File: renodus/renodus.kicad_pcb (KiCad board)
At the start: 4 copper layers, 40 x 40 mm, 67 parts, among them J1 USB_C_Receptacle_PowerOnly_6P, J2 Conn_01x02_Socket, J3 Conn_ARM_SWD_TagConnect_TC2030, SW1 SW_Push, SW2 SW_Push, U1 nRF54lxx_QDAA, U2 NPM1300-QEAA-R, U3 SHT4x, U4 STCC4, Y1 Crystal_GND24_Small, Y2 Crystal_Small

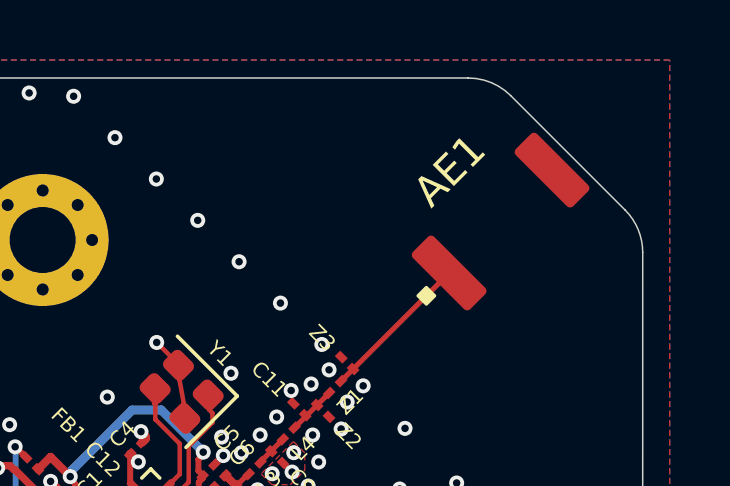
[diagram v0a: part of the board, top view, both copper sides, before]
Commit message: Small update
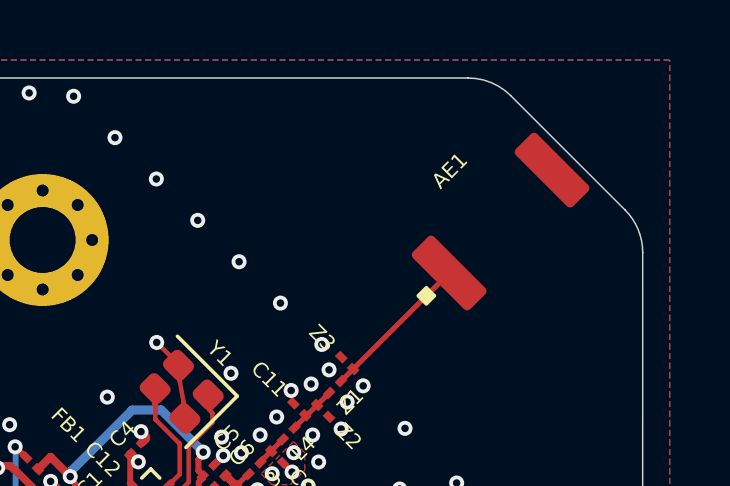
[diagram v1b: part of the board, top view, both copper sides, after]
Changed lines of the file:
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@@
 			(effects
 				(font
-					(size 1 1)
-					(thickness 0.15)
+					(size 0.5 0.5)
+					(thickness 0.125)
 				)
 			)
@@
 	)
 	(zone
-		(net "+3V0")
-		(layer "F.Cu")
-		(hatch none 0.1)
-		(priority 30000)
-		(attr
-			(teardrop
-				(type padvia)
-			)
-		)
-		(connect_pads yes
-			(clearance 0)
-		)
-		(min_thickness 0.0254)
-		(fill yes
-			(island_removal_mode 1)
-		)
-		(polygon
-			(pts
-				(xy 189.591794 106.341405) (xy 189.591794 106.741405) (xy 190.038217 106.786601) (xy 190.092794 106.541405)
-				(xy 190.038217 106.296209)
-			)
-		)
-	)
-	(zone
 		(layer "F.Cu")
 		(name "VBAT_BTM")
@@
 			)
 		)
+	)
+	(zone
+		(net "+3V0")
+		(layer "F.Cu")
+		(hatch none 0.1)
+		(priority 30000)
+		(attr
+			(teardrop
+				(type padvia)
+			)
+		)
+		(connect_pads yes
+			(clearance 0)
+		)
+		(min_thickness 0.0254)
+		(fill yes
+			(island_removal_mode 1)
+		)
+		(polygon
+			(pts
+				(xy 189.591794 106.341405) (xy 189.591794 106.741405) (xy 190.038217 106.786601) (xy 190.092794 106.541405)
+				(xy 190.038217 106.296209)
+			)
+		)
